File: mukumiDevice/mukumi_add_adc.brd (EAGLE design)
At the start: 49.2 x 43.9 mm, 157 parts, among them IC1 AD835, IC10 NJM2884, IC11 AD9834, IC12 AD9834, IC13 SIT8002B, IC14 NJM074V, IC2 AD835, IC3 MCP3422, IC5 NJM074V, IC6 NJM074V, IC7 NJM074V, IC8 NJM074V, IC9 NJM2884

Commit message: 部品表に0ohm抵抗が抜けていたのを訂正、メイン基板のサイズに合わせてユーティリティ基板のピンの位置、サイズの変更
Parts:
- C2, C3, C4, C56, C57, C58, C59: value 0.47u -> 1u
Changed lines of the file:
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@@
 <attribute name="VALUE" x="47.135" y="8.995" size="1.27" layer="28" rot="MR0"/>
 </element>
-<element name="C2" library="rcl" library_urn="urn:adsk.eagle:library:334" package="C1206" package3d_urn="urn:adsk.eagle:package:23618/2" value="0.47u" x="46.5" y="27.1" rot="MR90">
+<element name="C2" library="rcl" library_urn="urn:adsk.eagle:library:334" package="C1206" package3d_urn="urn:adsk.eagle:package:23618/2" value="1u" x="46.5" y="27.1" rot="MR90">
 <attribute name="SPICEPREFIX" value="C" x="46.5" y="27.1" size="1.778" layer="28" rot="MR90" display="off"/>
 </element>
-<element name="C3" library="rcl" library_urn="urn:adsk.eagle:library:334" package="C1206" package3d_urn="urn:adsk.eagle:package:23618/2" value="0.47u" x="20.7" y="19.4" rot="MR270">
+<element name="C3" library="rcl" library_urn="urn:adsk.eagle:library:334" package="C1206" package3d_urn="urn:adsk.eagle:package:23618/2" value="1u" x="20.7" y="19.4" rot="MR270">
 <attribute name="SPICEPREFIX" value="C" x="20.7" y="19.4" size="1.778" layer="28" rot="MR270" display="off"/>
 </element>
-<element name="C4" library="rcl" library_urn="urn:adsk.eagle:library:334" package="C1206" package3d_urn="urn:adsk.eagle:package:23618/2" value="0.47u" x="17.5" y="29.9" rot="MR90">
+<element name="C4" library="rcl" library_urn="urn:adsk.eagle:library:334" package="C1206" package3d_urn="urn:adsk.eagle:package:23618/2" value="1u" x="17.5" y="29.9" rot="MR90">
 <attribute name="SPICEPREFIX" value="C" x="17.5" y="29.9" size="1.778" layer="28" rot="MR90" display="off"/>
 </element>
@@
 <attribute name="SPICEPREFIX" value="C" x="34.8" y="25.6" size="1.778" layer="28" rot="MR180" display="off"/>
 </element>
-<element name="C56" library="rcl" library_urn="urn:adsk.eagle:library:334" package="C1206" package3d_urn="urn:adsk.eagle:package:23618/2" value="0.47u" x="27.2" y="15.4" rot="MR0">
+<element name="C56" library="rcl" library_urn="urn:adsk.eagle:library:334" package="C1206" package3d_urn="urn:adsk.eagle:package:23618/2" value="1u" x="27.2" y="15.4" rot="MR0">
 <attribute name="SPICEPREFIX" value="C" x="27.2" y="15.4" size="1.778" layer="28" rot="MR0" display="off"/>
 </element>
-<element name="C57" library="rcl" library_urn="urn:adsk.eagle:library:334" package="C1206" package3d_urn="urn:adsk.eagle:package:23618/2" value="0.47u" x="34.1" y="17.7" smashed="yes" rot="MR270">
+<element name="C57" library="rcl" library_urn="urn:adsk.eagle:library:334" package="C1206" package3d_urn="urn:adsk.eagle:package:23618/2" value="1u" x="34.1" y="17.7" smashed="yes" rot="MR270">
 <attribute name="NAME" x="32.83" y="18.97" size="1.27" layer="26" rot="MR270"/>
 <attribute name="SPICEPREFIX" value="C" x="34.1" y="17.7" size="1.778" layer="28" rot="MR270" display="off"/>
 <attribute name="VALUE" x="36.64" y="18.97" size="1.27" layer="28" rot="MR270"/>
 </element>
-<element name="C58" library="rcl" library_urn="urn:adsk.eagle:library:334" package="C1206" package3d_urn="urn:adsk.eagle:package:23618/2" value="0.47u" x="26.8" y="4.5" smashed="yes" rot="MR90">
+<element name="C58" library="rcl" library_urn="urn:adsk.eagle:library:334" package="C1206" package3d_urn="urn:adsk.eagle:package:23618/2" value="1u" x="26.8" y="4.5" smashed="yes" rot="MR90">
 <attribute name="NAME" x="27.97" y="2.53" size="1.27" layer="26" rot="MR90"/>
 <attribute name="SPICEPREFIX" value="C" x="26.8" y="4.5" size="1.778" layer="28" rot="MR90" display="off"/>
 <attribute name="VALUE" x="24.26" y="3.23" size="1.27" layer="28" rot="MR90"/>
 </element>
-<element name="C59" library="rcl" library_urn="urn:adsk.eagle:library:334" package="C1206" package3d_urn="urn:adsk.eagle:package:23618/2" value="0.47u" x="46.8" y="3.5" rot="MR90">
+<element name="C59" library="rcl" library_urn="urn:adsk.eagle:library:334" package="C1206" package3d_urn="urn:adsk.eagle:package:23618/2" value="1u" x="46.8" y="3.5" rot="MR90">
 <attribute name="SPICEPREFIX" value="C" x="46.8" y="3.5" size="1.778" layer="28" rot="MR90" display="off"/>
 </element>

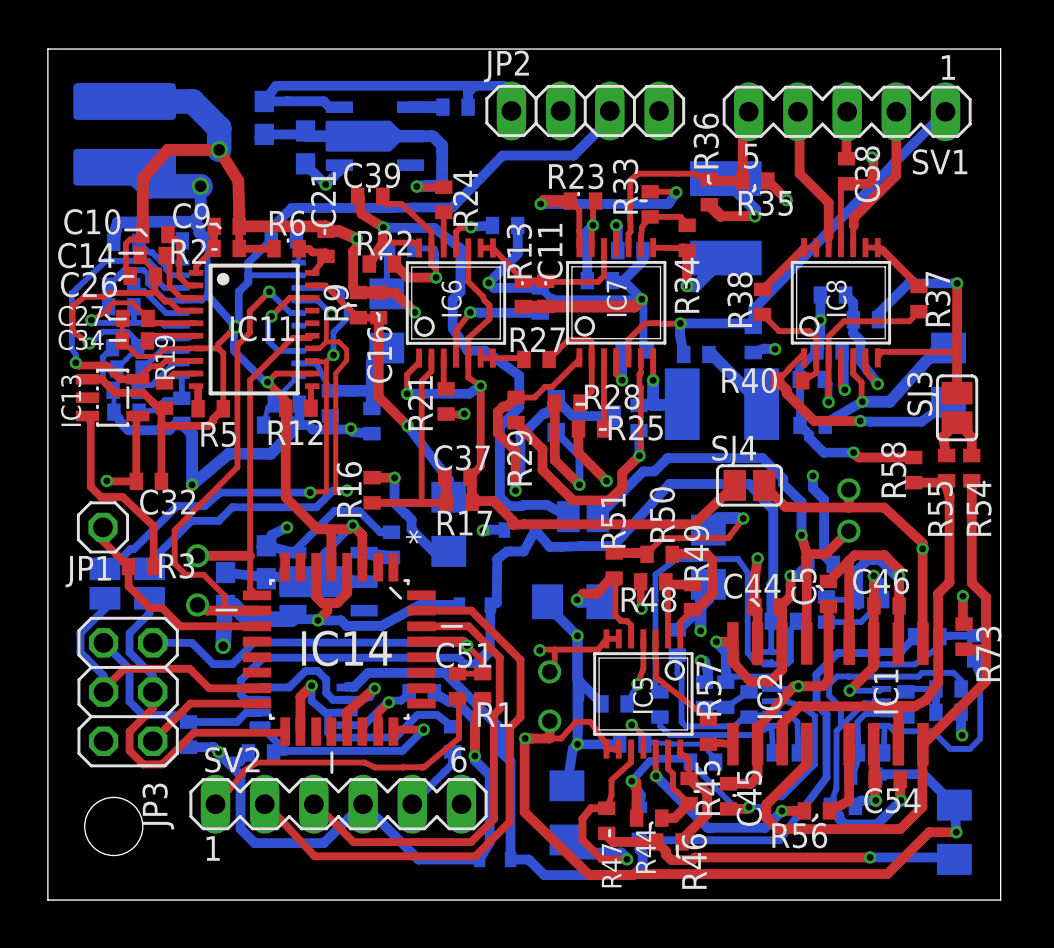
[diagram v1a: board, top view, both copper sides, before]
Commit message: P板からの指摘点を修正、ad633用ユーティリティ基板の作成
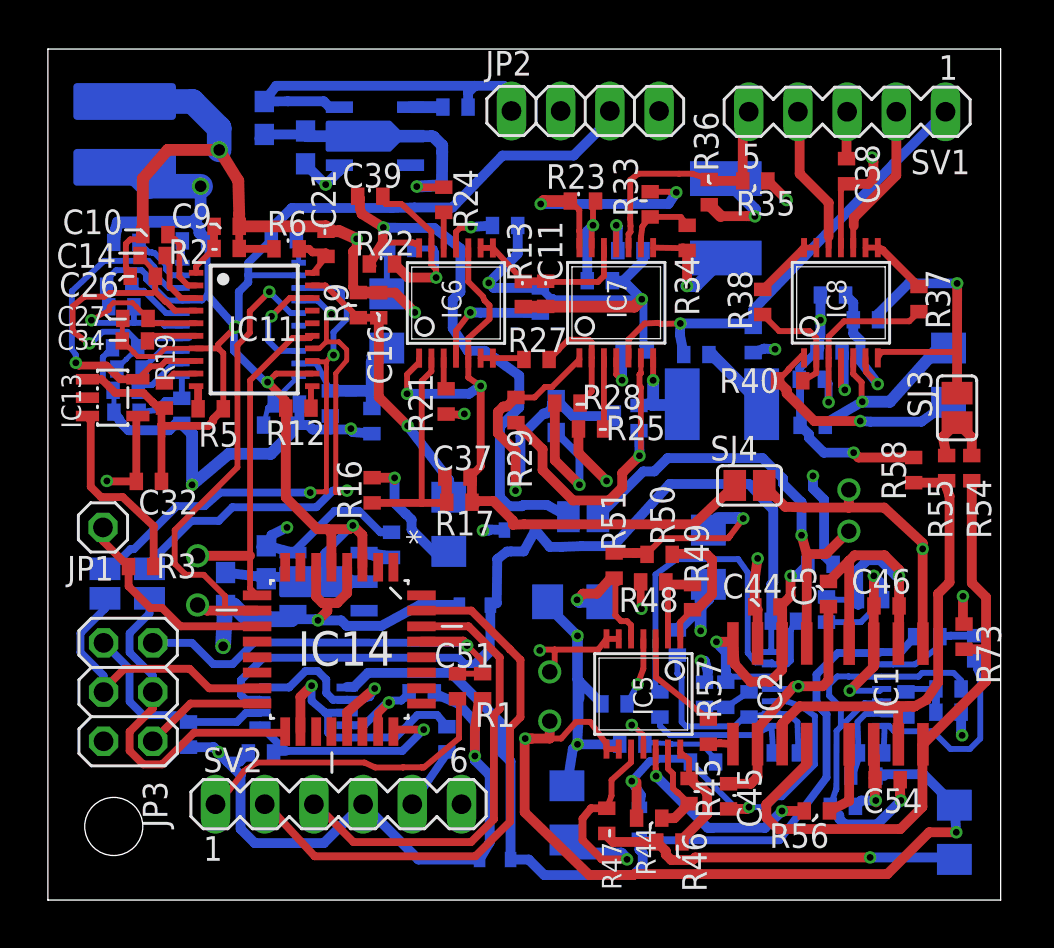
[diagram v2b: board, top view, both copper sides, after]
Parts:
- R44, R48: value 560 -> 4.7k
- moved C7 0.30 mm to (20.6, 8.30)
- moved C13 0.10 mm to (3.68, 31.7)
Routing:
- net AGND: track 411.0 -> 413.4 mm
